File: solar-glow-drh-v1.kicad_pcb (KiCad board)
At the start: 4 copper layers, 50.8 x 88.9 mm, 37 parts, among them SW1 SW_F12340, SW2 slide OFF/ON/TINY

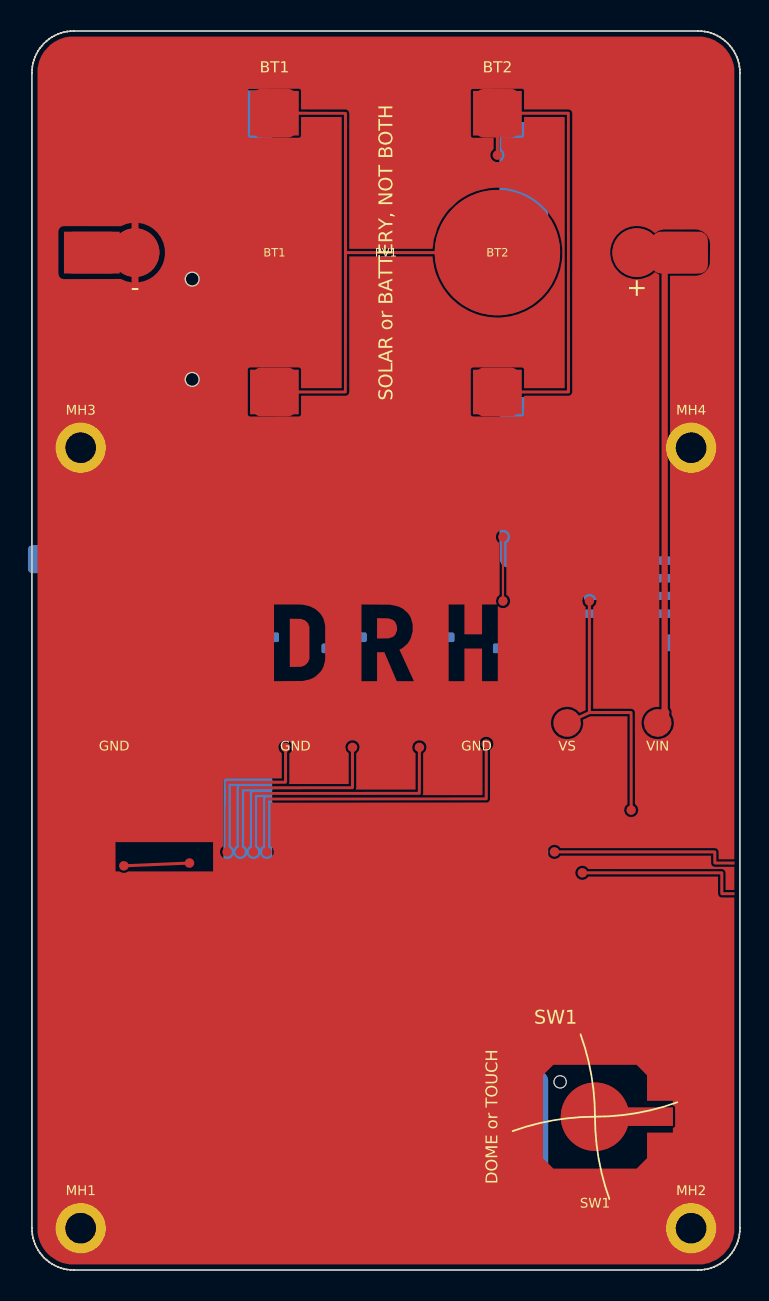
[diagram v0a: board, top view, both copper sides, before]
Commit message: Add files via upload
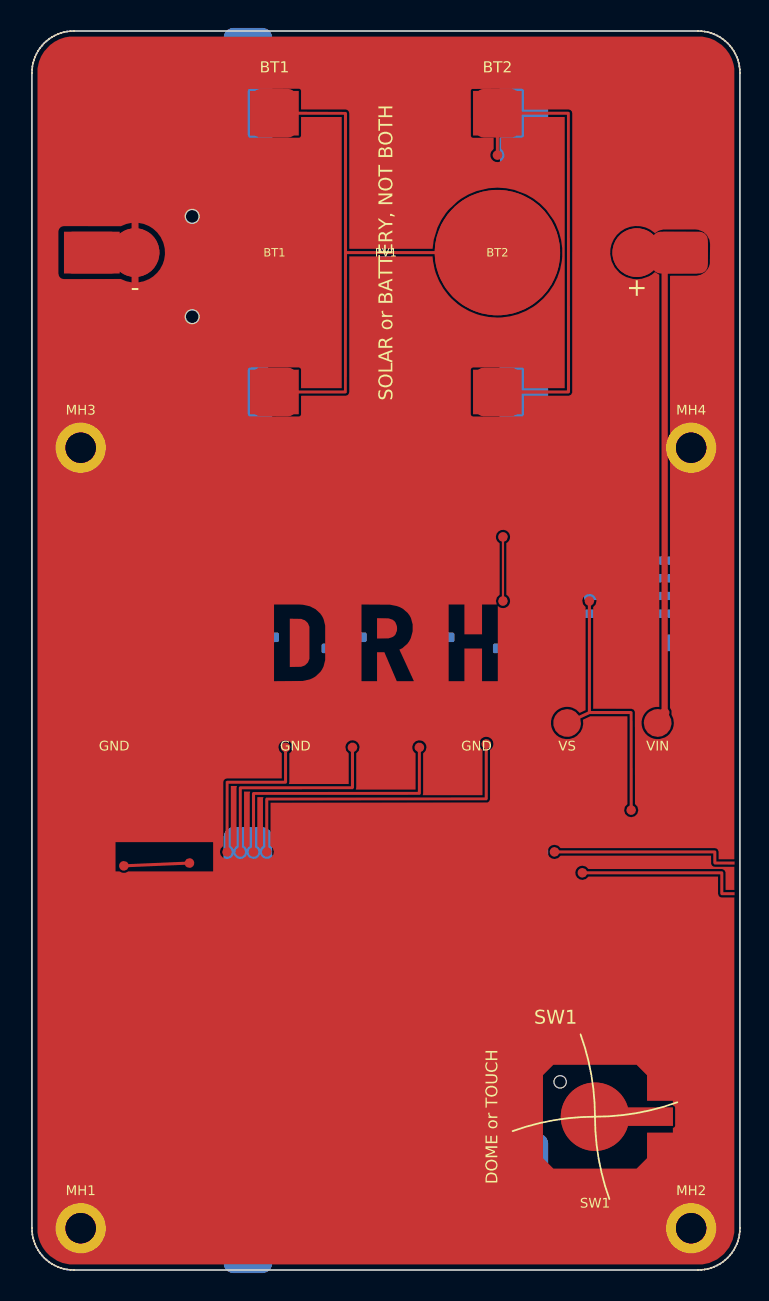
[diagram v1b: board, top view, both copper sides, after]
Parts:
- added ACCEL?: , M1:ACCEL_reserved, B.Cu at (20.0, 35.9)
- added JP2: , JP2:HDR1x4, B.Cu at (6.00, 54.9)
- SW2: value slide OFF/ON/TINY -> (none); footprint slide_OFF/ON/TINY -> SW2:SJ_3way
- moved SW2 33.7 mm to (11.7, 53.9)
- moved C3 7.18 mm to (5.00, 45.5)
- moved C4 5.89 mm to (43.0, 36.1)
- moved C1 4.78 mm to (9.50, 45.5)
- moved C5 4.66 mm to (8.20, 50.4)
- moved R5 4.66 mm to (4.20, 50.4)
- moved R6 4.66 mm to (6.20, 50.4)
- moved SC1 4.50 mm to (15.5, 16.9)
- moved SC2 4.50 mm to (35.3, 16.9)
- moved SC3 4.50 mm to (15.5, 72.0)
- moved SC4 4.50 mm to (35.3, 72.0)
- moved TC1 4.50 mm to (11.5, 16.9)
- moved SJ1 3.21 mm to (13.2, 45.1)
- moved C2 1.98 mm to (9.50, 36.6)
- moved J1 1.77 mm to (4.70, 38.4), turned to 0 degrees
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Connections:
- U1 pad 2: (no net) -> PA4
- U1 pad 22: RESET -> (no net)
- U1 pad 6: (no net) -> PC0
- U1 pad 7: (no net) -> PC1
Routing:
- added copper zone on In1.Cu, net GND
- added copper zone on In2.Cu, net VS
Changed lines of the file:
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@@
   (net 11 "LDRV4")
   (net 12 "MID")
-  (net 13 "RESET")
   (net 14 "SCL")
   (net 15 "SDA")
@@
   (net 22 "VS")
   (net 23 "VSENSE")
+  (net 24 "PA4")
+  (net 25 "PC0")
+  (net 26 "PC1")
   (footprint "MountingHole_M2_2.2mm" (layer "F.Cu")
     (at 3.5 85.9)
@@
       (net 1 "GND") (solder_mask_margin -0.1))
   )
-  (footprint "slide_OFF/ON/TINY" (layer "B.Cu")
-    (at 25.0 84.9 0)
-    (attr smd)
-    (fp_rect (start -3.3 -1.5) (end 3.3 1.5) (layer "B.CrtYd") (width 0.05) (fill none))
-    (fp_text reference "SW2" (at 0 0 0) (layer "B.SilkS")
-      (effects (font (size 0.7 0.7) (thickness 0.12)))
-    )
-    (fp_text value "slide OFF/ON/TINY" (at 0 2.2 0) (layer "B.Fab")
-      (effects (font (size 0.5 0.5) (thickness 0.1)))
-    )
-  )
   (footprint "TC2030-IDC-NL" (layer "B.Cu")
-    (at 11.5 21.4)
+    (at 11.5 16.9)
     (attr smd exclude_from_bom)
     (fp_rect (start -3 -4.95) (end 3 4.95) (layer "B.CrtYd") (width 0.05) (fill none))
@@
   )
   (footprint "SC1:SCPC" (layer "B.Cu")
-    (at 15.5 21.4 90)
+    (at 15.5 16.9 90)
     (attr smd)
     (fp_rect (start -14.25 -8.5) (end 14.25 8.5) (layer "B.CrtYd") (width 0.05) (fill none))
@@
   )
   (footprint "SC2:SCPC" (layer "B.Cu")
-    (at 35.3 21.4 270)
+    (at 35.3 16.9 270)
     (attr smd)
     (fp_rect (start -14.25 -8.5) (end 14.25 8.5) (layer "B.CrtYd") (width 0.05) (fill none))
@@
   )
   (footprint "SC3:SCPC" (layer "B.Cu")
-    (at 15.5 67.5 270)
+    (at 15.5 72 270)
     (attr smd)
     (fp_rect (start -14.25 -8.5) (end 14.25 8.5) (layer "B.CrtYd") (width 0.05) (fill none))
@@
   )
   (footprint "SC4:SCPC" (layer "B.Cu")
-    (at 35.3 67.5 90)
+    (at 35.3 72 90)
     (attr smd)
     (fp_rect (start -14.25 -8.5) (end 14.25 8.5) (layer "B.CrtYd") (width 0.05) (fill none))
@@
       (net 11 "LDRV4"))
     (pad "2" smd roundrect (at -2 -0.8) (size 0.8 0.2) (layers "B.Cu" "B.Mask" "B.Paste") (roundrect_rratio 0.2)
-      (net 0 ""))
+      (net 24 "PA4"))
     (pad "3" smd roundrect (at -2 -0.4) (size 0.8 0.2) (layers "B.Cu" "B.Mask" "B.Paste") (roundrect_rratio 0.2)
       (net 23 "VSENSE"))
@@
       (net 3 "BTN"))
     (pad "6" smd roundrect (at -2 0.8) (size 0.8 0.2) (layers "B.Cu" "B.Mask" "B.Paste") (roundrect_rratio 0.2)
-      (net 0 ""))
+      (net 25 "PC0"))
     (pad "7" smd roundrect (at -2 1.2) (size 0.8 0.2) (layers "B.Cu" "B.Mask" "B.Paste") (roundrect_rratio 0.2)
-      (net 0 ""))
+      (net 26 "PC1"))
     (pad "8" smd roundrect (at -1.2 2) (size 0.2 0.8) (layers "B.Cu" "B.Mask" "B.Paste") (roundrect_rratio 0.2)
       (net 15 "SDA"))
@@
       (net 0 ""))
     (pad "22" smd roundrect (at 1.2 -2) (size 0.2 0.8) (layers "B.Cu" "B.Mask" "B.Paste") (roundrect_rratio 0.2)
-      (net 13 "RESET"))
+      (net 0 ""))
     (pad "23" smd roundrect (at 0.8 -2) (size 0.2 0.8) (layers "B.Cu" "B.Mask" "B.Paste") (roundrect_rratio 0.2)
       (net 17 "UPDI"))
@@
   )
   (footprint "U2:SOIC8" (layer "B.Cu")
-    (at 43.0 39.9 0)
+    (at 43 39.9 0)
     (attr smd)
     (fp_rect (start -2.45 -1.95) (end 2.45 1.95) (layer "B.CrtYd") (width 0.05) (fill none))
@@
   )
   (footprint "D1:SOD" (layer "B.Cu")
-    (at 44.0 43.9 0)
+    (at 44 43.9 0)
     (attr smd)
     (fp_rect (start -1.85 -0.8) (end 1.85 0.8) (layer "B.CrtYd") (width 0.05) (fill none))
@@
   )
   (footprint "C1:0805" (layer "B.Cu")
-    (at 5.0 43.9 0)
+    (at 9.5 45.5 0)
     (attr smd)
     (fp_rect (start -1 -0.625) (end 1 0.625) (layer "B.CrtYd") (width 0.05) (fill none))
@@
   )
   (footprint "C2:0805" (layer "B.Cu")
-    (at 8.0 37.9 0)
+    (at 9.5 36.6 0)
     (attr smd)
     (fp_rect (start -1 -0.625) (end 1 0.625) (layer "B.CrtYd") (width 0.05) (fill none))
@@
   )
   (footprint "C3:0805" (layer "B.Cu")
-    (at 12.0 43.9 0)
+    (at 5 45.5 0)
     (attr smd)
     (fp_rect (start -1 -0.625) (end 1 0.625) (layer "B.CrtYd") (width 0.05) (fill none))
@@
   )
   (footprint "C4:0402" (layer "B.Cu")
-    (at 47.5 39.9 0)
+    (at 43 36.1 0)
     (attr smd)
     (fp_rect (start -0.5 -0.25) (end 0.5 0.25) (layer "B.CrtYd") (width 0.05) (fill none))
@@
   )
   (footprint "J1:PROG" (layer "B.Cu")
-    (at 3.0 37.9 90)
+    (at 4.7 38.4 0)
     (attr smd)
     (fp_text reference "J1" (at 0 0 0) (layer "B.SilkS")
@@
   )
   (footprint "JP1:PROG" (layer "B.Cu")
-    (at 13.5 37.9 90)
+    (at 13.7 38.9 0)
     (attr smd)
     (fp_text reference "JP1" (at 0 0 0) (layer "B.SilkS")
@@
   )
   (footprint "SJ1:0402" (layer "B.Cu")
-    (at 13.0 41.9 0)
+    (at 13.2 45.1 0)
     (attr smd)
     (fp_rect (start -0.5 -0.25) (end 0.5 0.25) (layer "B.CrtYd") (width 0.05) (fill none))
@@
   )
   (footprint "R5:0402" (layer "B.Cu")
-    (at 3.0 45.9 0)
+    (at 4.2 50.4 0)
     (attr smd)
     (fp_rect (start -0.5 -0.25) (end 0.5 0.25) (layer "B.CrtYd") (width 0.05) (fill none))
@@
   )
   (footprint "R6:0402" (layer "B.Cu")
-    (at 5.0 45.9 0)
+    (at 6.2 50.4 0)
     (attr smd)
     (fp_rect (start -0.5 -0.25) (end 0.5 0.25) (layer "B.CrtYd") (width 0.05) (fill none))
@@
   )
   (footprint "C5:0402" (layer "B.Cu")
-    (at 7.0 45.9 0)
+    (at 8.2 50.4 0)
     (attr smd)
     (fp_rect (start -0.5 -0.25) (end 0.5 0.25) (layer "B.CrtYd") (width 0.05) (fill none))
@@
       (net 1 "GND"))
   )
+  (footprint "JP2:HDR1x4" (layer "B.Cu")
+    (at 6 54.9 0)
+    (attr smd)
+    (fp_rect (start -2.5 -1.25) (end 2.5 1.25) (layer "B.CrtYd") (width 0.05) (fill none))
+    (fp_text reference "JP2" (at 0 0 0) (layer "B.SilkS")
+      (effects (font (size 0.5 0.5) (thickness 0.08)))
+    )
+    (pad "1" smd roundrect (at -1.905 0) (size 0.9 1.5) (layers "B.Cu" "B.Mask" "B.Paste") (roundrect_rratio 0.25)
+      (net 24 "PA4"))
+    (pad "2" smd roundrect (at -0.635 0) (size 0.9 1.5) (layers "B.Cu" "B.Mask" "B.Paste") (roundrect_rratio 0.25)
+      (net 25 "PC0"))
+    (pad "3" smd roundrect (at 0.635 0) (size 0.9 1.5) (layers "B.Cu" "B.Mask" "B.Paste") (roundrect_rratio 0.25)
+      (net 26 "PC1"))
+    (pad "4" smd roundrect (at 1.905 0) (size 0.9 1.5) (layers "B.Cu" "B.Mask" "B.Paste") (roundrect_rratio 0.25)
+      (net 1 "GND"))
+  )
+  (footprint "SW2:SJ_3way" (layer "B.Cu")
+    (at 11.7 53.9 0)
+    (attr smd)
+    (fp_rect (start -2.25 -1.1) (end 2.25 1.1) (layer "B.CrtYd") (width 0.05) (fill none))
+    (fp_text reference "SW2" (at 0 0 0) (layer "B.SilkS")
+      (effects (font (size 0.5 0.5) (thickness 0.08)))
+    )
+    (pad "1" smd roundrect (at -1.4 0) (size 1 1.4) (layers "B.Cu" "B.Mask" "B.Paste") (roundrect_rratio 0.2)
+      (net 0 ""))
+    (pad "2" smd roundrect (at 0 0) (size 1 1.4) (layers "B.Cu" "B.Mask" "B.Paste") (roundrect_rratio 0.2)
+      (net 0 ""))
+    (pad "3" smd roundrect (at 1.4 0) (size 1 1.4) (layers "B.Cu" "B.Mask" "B.Paste") (roundrect_rratio 0.2)
+      (net 0 ""))
+  )
+  (footprint "M1:ACCEL_reserved" (layer "B.Cu")
+    (at 20 35.9 0)
+    (attr smd)
+    (fp_rect (start -1.75 -1.75) (end 1.75 1.75) (layer "B.CrtYd") (width 0.05) (fill none))
+    (fp_text reference "ACCEL?" (at 0 0 0) (layer "B.SilkS")
+      (effects (font (size 0.5 0.5) (thickness 0.08)))
+    )
+    (pad "x" smd roundrect (at -1 -1) (size 0.5 0.5) (layers "B.Cu" "B.Mask" "B.Paste") (roundrect_rratio 0.25)
+      (net 0 ""))
+    (pad "x" smd roundrect (at 1 -1) (size 0.5 0.5) (layers "B.Cu" "B.Mask" "B.Paste") (roundrect_rratio 0.25)
+      (net 0 ""))
+    (pad "x" smd roundrect (at 1 1) (size 0.5 0.5) (layers "B.Cu" "B.Mask" "B.Paste") (roundrect_rratio 0.25)
+      (net 0 ""))
+    (pad "x" smd roundrect (at -1 1) (size 0.5 0.5) (layers "B.Cu" "B.Mask" "B.Paste") (roundrect_rratio 0.25)
+      (net 0 ""))
+  )
   (gr_poly
     (pts
@@
   (gr_circle (center 28.6544 43.9) (end 29.4744 43.9) (layer "B.Cu") (width 0.1) (fill none))
   (gr_circle (center 34.6781 43.9) (end 35.4981 43.9) (layer "B.Cu") (width 0.1) (fill none))
+  (zone (net 1) (net_name "GND") (layer "In1.Cu") (hatch edge 0.508)
+    (connect_pads thermal_relief (clearance 0.254))
+    (min_thickness 0.2)
+    (fill yes (thermal_gap 0.2) (thermal_bridge_width 0.25))
+    (polygon
+      (pts
+        (xy 0 0)
+        (xy 50.8 0)
+        (xy 50.8 88.9)
+        (xy 0 88.9)
+      )
+    )
+  )
+  (zone (net 22) (net_name "VS") (layer "In2.Cu") (hatch edge 0.508)
+    (connect_pads thermal_relief (clearance 0.254))
+    (min_thickness 0.2)
+    (fill yes (thermal_gap 0.2) (thermal_bridge_width 0.25))
+    (polygon
+      (pts
+        (xy 0 0)
+        (xy 50.8 0)
+        (xy 50.8 88.9)
+        (xy 0 88.9)
+      )
+    )
+  )
+  (zone (net 0) (net_name "") (layers "F.Cu" "In1.Cu" "In2.Cu" "B.Cu") (name "glow_keepout") (hatch edge 0.508)
+    (connect_pads (clearance 0.254))
+    (min_thickness 0.254)
+    (keepout (tracks allowed) (vias not_allowed) (pads allowed ) (copperpour not_allowed) (footprints not_allowed))
+    (polygon
+      (pts
+        (xy 14.95 40.8)
+        (xy 35.849999999999994 40.8)
+        (xy 35.849999999999994 47)
+        (xy 14.95 47)
+      )
+    )
+  )
 )

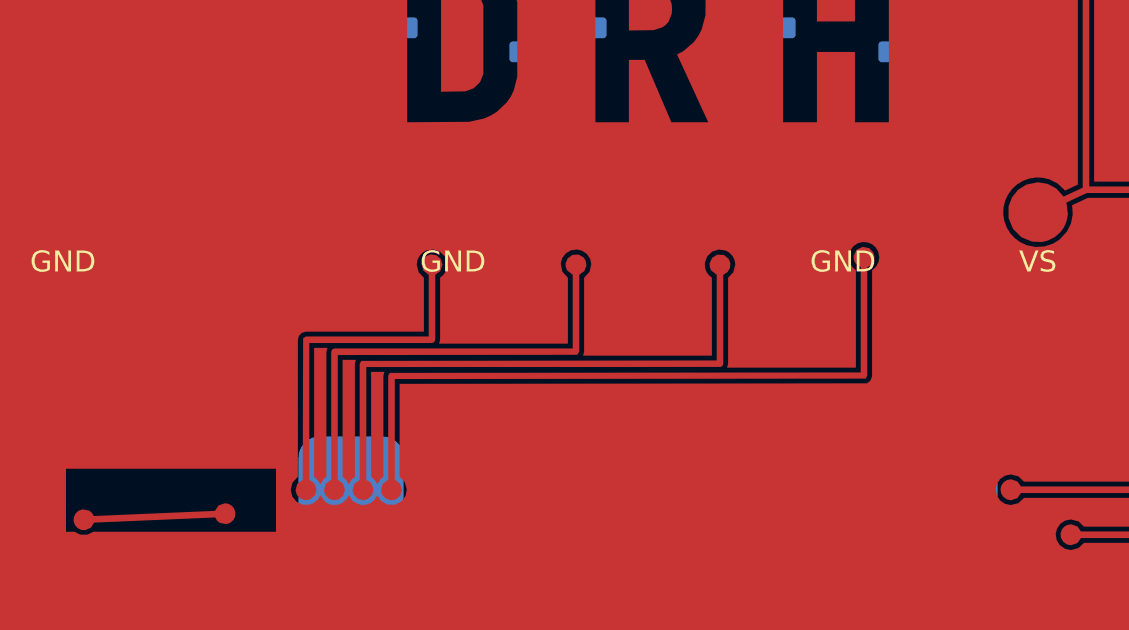
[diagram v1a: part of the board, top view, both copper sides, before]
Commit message: Add files via upload
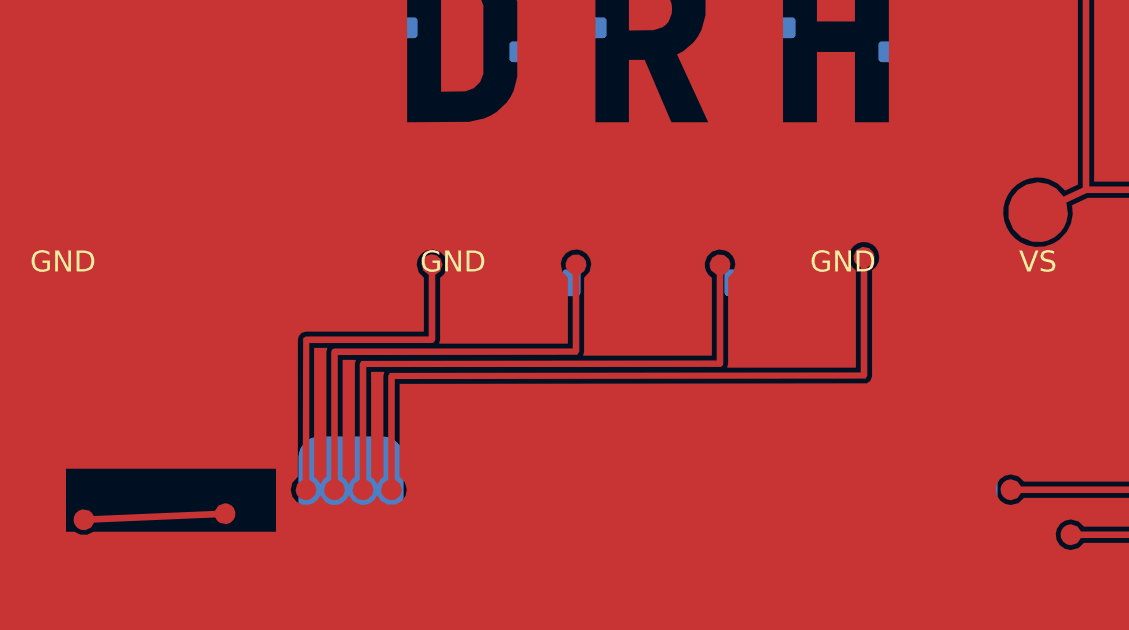
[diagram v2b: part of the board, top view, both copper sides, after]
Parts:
- removed ACCEL?: , M1:ACCEL_reserved
- removed SW2: , SW2:SJ_3way
- added M1: , M1:ACCEL_reserved, B.Cu at (20.0, 35.9)
- added SB1: , SB1:bridge_2pad, B.Cu at (16.1, 52.0)
- added SB2: , SB2:bridge_2pad, B.Cu at (22.4, 52.0)
- added SB3: , SB3:bridge_2pad, B.Cu at (28.7, 52.0)
- added SB4: , SB4:bridge_2pad, B.Cu at (34.7, 52.0)
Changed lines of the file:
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@@
   (net 14 "SCL")
   (net 15 "SDA")
-  (net 16 "TBD_SW2")
   (net 17 "UPDI")
   (net 18 "VBAT")
@@
       (net 1 "GND"))
   )
-  (footprint "SW2:SJ_3way" (layer "B.Cu")
-    (at 11.7 53.9 0)
-    (attr smd)
-    (fp_rect (start -2.25 -1.1) (end 2.25 1.1) (layer "B.CrtYd") (width 0.05) (fill none))
-    (fp_text reference "SW2" (at 0 0 0) (layer "B.SilkS")
-      (effects (font (size 0.5 0.5) (thickness 0.08)))
-    )
-    (pad "1" smd roundrect (at -1.4 0) (size 1 1.4) (layers "B.Cu" "B.Mask" "B.Paste") (roundrect_rratio 0.2)
-      (net 0 ""))
-    (pad "2" smd roundrect (at 0 0) (size 1 1.4) (layers "B.Cu" "B.Mask" "B.Paste") (roundrect_rratio 0.2)
-      (net 0 ""))
-    (pad "3" smd roundrect (at 1.4 0) (size 1 1.4) (layers "B.Cu" "B.Mask" "B.Paste") (roundrect_rratio 0.2)
-      (net 0 ""))
+  (footprint "SB1:bridge_2pad" (layer "B.Cu")
+    (at 16.1 52.0 0)
+    (attr smd)
+    (fp_rect (start -0.95 -0.65) (end 0.95 0.65) (layer "B.CrtYd") (width 0.05) (fill none))
+    (fp_text reference "SB1" (at 0 -1.15 0) (layer "B.SilkS")
+      (effects (font (size 0.5 0.5) (thickness 0.08)))
+    )
+    (pad "1" smd roundrect (at -0.45 0) (size 0.6 0.9) (layers "B.Cu" "B.Mask" "B.Paste") (roundrect_rratio 0.2)
+      (net 8 "LDRV1"))
+    (pad "2" smd roundrect (at 0.45 0) (size 0.6 0.9) (layers "B.Cu" "B.Mask" "B.Paste") (roundrect_rratio 0.2)
+      (net 1 "GND"))
+  )
+  (footprint "SB2:bridge_2pad" (layer "B.Cu")
+    (at 22.4 52.0 0)
+    (attr smd)
+    (fp_rect (start -0.95 -0.65) (end 0.95 0.65) (layer "B.CrtYd") (width 0.05) (fill none))
+    (fp_text reference "SB2" (at 0 -1.15 0) (layer "B.SilkS")
+      (effects (font (size 0.5 0.5) (thickness 0.08)))
+    )
+    (pad "1" smd roundrect (at -0.45 0) (size 0.6 0.9) (layers "B.Cu" "B.Mask" "B.Paste") (roundrect_rratio 0.2)
+      (net 9 "LDRV2"))
+    (pad "2" smd roundrect (at 0.45 0) (size 0.6 0.9) (layers "B.Cu" "B.Mask" "B.Paste") (roundrect_rratio 0.2)
+      (net 1 "GND"))
+  )
+  (footprint "SB3:bridge_2pad" (layer "B.Cu")
+    (at 28.7 52.0 0)
+    (attr smd)
+    (fp_rect (start -0.95 -0.65) (end 0.95 0.65) (layer "B.CrtYd") (width 0.05) (fill none))
+    (fp_text reference "SB3" (at 0 -1.15 0) (layer "B.SilkS")
+      (effects (font (size 0.5 0.5) (thickness 0.08)))
+    )
+    (pad "1" smd roundrect (at -0.45 0) (size 0.6 0.9) (layers "B.Cu" "B.Mask" "B.Paste") (roundrect_rratio 0.2)
+      (net 10 "LDRV3"))
+    (pad "2" smd roundrect (at 0.45 0) (size 0.6 0.9) (layers "B.Cu" "B.Mask" "B.Paste") (roundrect_rratio 0.2)
+      (net 1 "GND"))
+  )
+  (footprint "SB4:bridge_2pad" (layer "B.Cu")
+    (at 34.7 52.0 0)
+    (attr smd)
+    (fp_rect (start -0.95 -0.65) (end 0.95 0.65) (layer "B.CrtYd") (width 0.05) (fill none))
+    (fp_text reference "SB4" (at 0 -1.15 0) (layer "B.SilkS")
+      (effects (font (size 0.5 0.5) (thickness 0.08)))
+    )
+    (pad "1" smd roundrect (at -0.45 0) (size 0.6 0.9) (layers "B.Cu" "B.Mask" "B.Paste") (roundrect_rratio 0.2)
+      (net 11 "LDRV4"))
+    (pad "2" smd roundrect (at 0.45 0) (size 0.6 0.9) (layers "B.Cu" "B.Mask" "B.Paste") (roundrect_rratio 0.2)
+      (net 1 "GND"))
   )
   (footprint "M1:ACCEL_reserved" (layer "B.Cu")
@@
     (attr smd)
     (fp_rect (start -1.75 -1.75) (end 1.75 1.75) (layer "B.CrtYd") (width 0.05) (fill none))
-    (fp_text reference "ACCEL?" (at 0 0 0) (layer "B.SilkS")
-      (effects (font (size 0.5 0.5) (thickness 0.08)))
-    )
+    (fp_text reference "M1" (at 0 0 0) (layer "B.SilkS")
+      (effects (font (size 0.5 0.5) (thickness 0.08)))
+    )
